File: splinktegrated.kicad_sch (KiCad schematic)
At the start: 55 parts, among them J1 USB_C_Receptacle_USB2.0, J10 NA_Ribbon, J11 NA_Serial, J12 NA_Conn_01x04_Female, J13 Conn_01x02_Female, J14 Cirque, J2 NA_Conn_01x04_Female, J3 NA_Conn_01x04_Female, J4 NA_Conn_01x04_Female, J5 Conn_01x02, J7 NA_trackball, J8 NA_Ribbon, J9 NA_RGB, SW1 NA_SW_SPST, SW2 NA_SW_SPST, U1 RP2040, U2 USBLC6-2P6, U3 XC6210B332MR-G, U4 USBLC6-2P6, U5 W25Q128JVS, Y1 Crystal_GND24

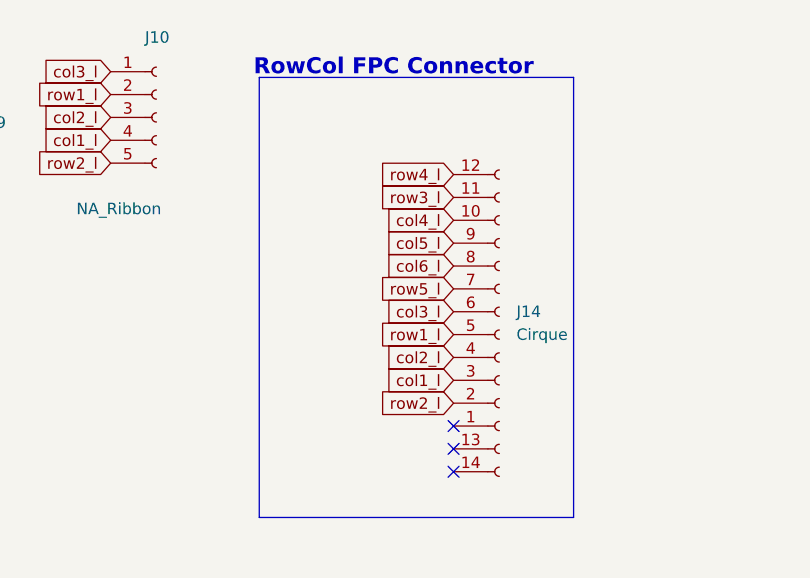
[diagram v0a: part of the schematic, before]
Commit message: routin
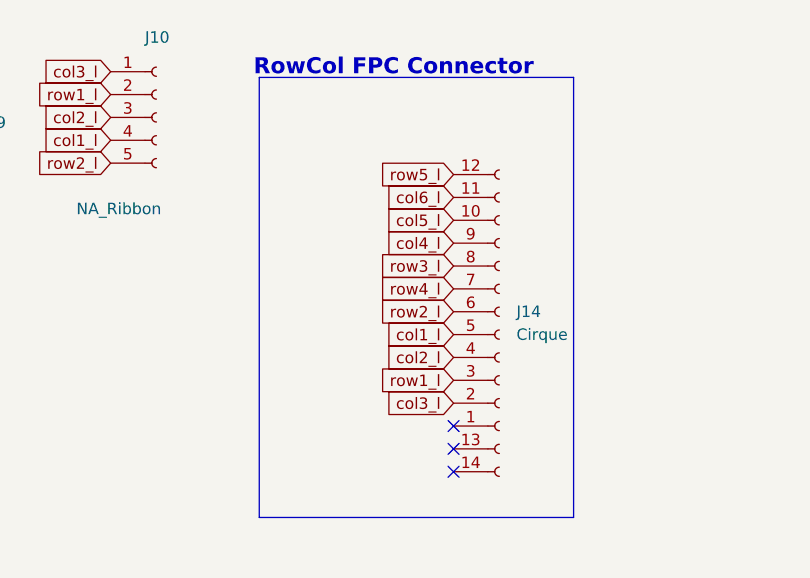
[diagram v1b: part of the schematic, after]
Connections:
- net col1_l: now also J14.5 (Pin_5); no longer J14.3 (Pin_3)
- net col3_l: now also J14.2 (Pin_2); no longer J14.6 (Pin_6)
- net col4_l: now also J14.9 (Pin_9); no longer J14.10 (Pin_10)
- net col5_l: now also J14.10 (Pin_10); no longer J14.9 (Pin_9)
- net col6_l: now also J14.11 (Pin_11); no longer J14.8 (Pin_8)
- net row1_l: now also J14.3 (Pin_3); no longer J14.5 (Pin_5)
- net row2_l: now also J14.6 (Pin_6); no longer J14.2 (Pin_2)
- net row3_l: now also J14.8 (Pin_8); no longer J14.11 (Pin_11)
- net row4_l: now also J14.7 (Pin_7); no longer J14.12 (Pin_12)
- net row5_l: now also J14.12 (Pin_12); no longer J14.7 (Pin_7)
